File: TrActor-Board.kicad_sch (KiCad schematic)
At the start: 24 parts, among them J3 GCT4720, J4 Batt, J5 NTC, SW1 Power, SW2 Reset, U3 LSM6DSO32, U6 USBLC6-2P6

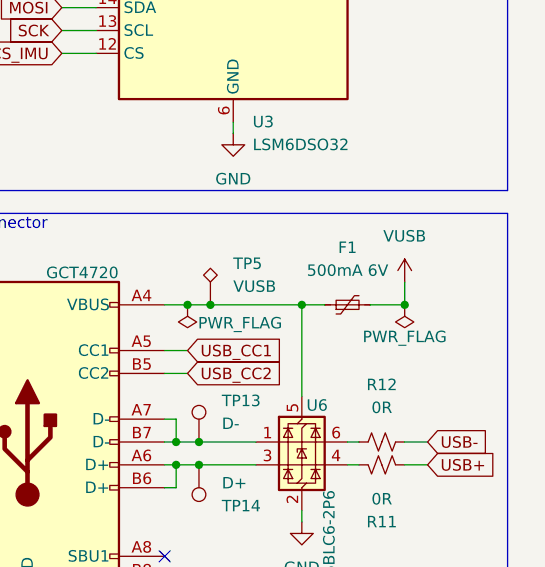
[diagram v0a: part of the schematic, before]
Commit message: routing started
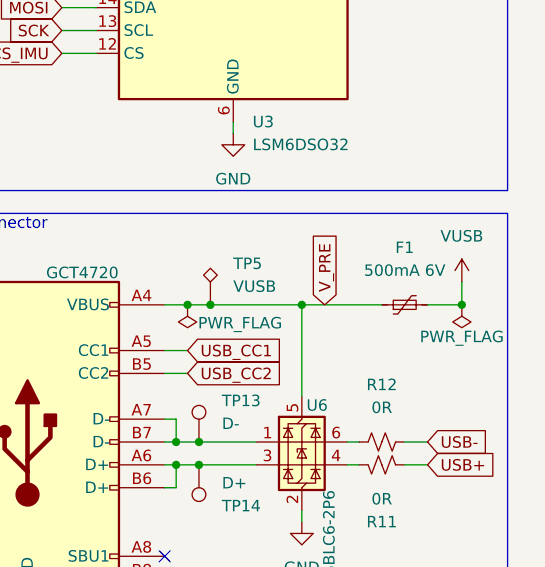
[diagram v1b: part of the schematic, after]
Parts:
- J5: footprint (none) -> Connector_JST:JST_SH_SM02B-SRSS-TB_1x02-1MP_P1.00mm_Horizontal
- JP1: footprint (none) -> Connector_PinHeader_2.54mm:PinHeader_1x02_P2.54mm_Vertical_SMD_Pin1Left
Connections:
- net V_PRE: now reaches F1.1, J3.A4 (VBUS), J3.A9 (VBUS), J3.B4 (VBUS), J3.B9 (VBUS), TP5.1, U6.5 (VBUS)
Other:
- moved on the sheet: F1
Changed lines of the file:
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@@
 	)
 	(junction
-		(at 252.73 82.55)
+		(at 259.08 82.55)
 		(diameter 0)
 		(color 0 0 0 0)
@@
 	)
 	(junction
+		(at 241.3 82.55)
+		(diameter 0)
+		(color 0 0 0 0)
+	)
+	(junction
 		(at 181.61 64.77)
 		(diameter 0)
@@
 	)
 	(junction
-		(at 241.3 82.55)
-		(diameter 0)
-		(color 0 0 0 0)
-	)
-	(junction
 		(at 191.77 64.77)
 		(diameter 0)
@@
 	(wire
 		(pts
-			(xy 252.73 82.55) (xy 248.92 82.55)
+			(xy 259.08 82.55) (xy 255.27 82.55)
 		)
 		(stroke
@@
 	(wire
 		(pts
-			(xy 243.84 82.55) (xy 241.3 82.55)
-		)
-		(stroke
-			(width 0)
-			(type default)
-		)
-	)
-	(wire
-		(pts
 			(xy 185.42 33.02) (xy 185.42 31.75)
 		)
@@
 	(wire
 		(pts
+			(xy 241.3 82.55) (xy 250.19 82.55)
+		)
+		(stroke
+			(width 0)
+			(type default)
+		)
+	)
+	(wire
+		(pts
 			(xy 172.72 78.74) (xy 176.53 78.74)
 		)
@@
 	(wire
 		(pts
-			(xy 252.73 80.01) (xy 252.73 82.55)
+			(xy 259.08 80.01) (xy 259.08 82.55)
 		)
 		(stroke
@@
 		)
 	)
+	(global_label "V_PRE"
+		(shape input)
+		(at 243.84 82.55 90)
+		(fields_autoplaced yes)
+		(effects
+			(font
+				(size 1.27 1.27)
+			)
+			(justify left)
+		)
+		(property "Intersheetrefs" "${INTERSHEET_REFS}"
+			(at 243.84 74.4738 90)
+			(hide yes)
+			(show_name no)
+			(do_not_autoplace no)
+			(effects
+				(font
+					(size 1.27 1.27)
+				)
+				(justify left)
+			)
+		)
+	)
 	(global_label "IMU_INT2"
 		(shape input)
@@
 	(symbol
 		(lib_id "power:VBUS")
-		(at 252.73 80.01 0)
+		(at 259.08 80.01 0)
 		(unit 1)
 		(body_style 1)
@@
 		(fields_autoplaced yes)
 		(property "Reference" "#PWR060"
-			(at 252.73 83.82 0)
+			(at 259.08 83.82 0)
 			(hide yes)
 			(show_name no)
@@
 		)
 		(property "Value" "VUSB"
-			(at 252.73 74.93 0)
+			(at 259.08 74.93 0)
 			(show_name no)
 			(do_not_autoplace no)
@@
 		)
 		(property "Footprint" ""
-			(at 252.73 80.01 0)
+			(at 259.08 80.01 0)
 			(hide yes)
 			(show_name no)
@@
 		)
 		(property "Datasheet" ""
-			(at 252.73 80.01 0)
+			(at 259.08 80.01 0)
 			(hide yes)
 			(show_name no)
@@
 		)
 		(property "Description" "Power symbol creates a global label with name \"VBUS\""
-			(at 252.73 80.01 0)
+			(at 259.08 80.01 0)
 			(hide yes)
 			(show_name no)
@@
 			)
 		)
-		(property "Footprint" ""
+		(property "Footprint" "Connector_JST:JST_SH_SM02B-SRSS-TB_1x02-1MP_P1.00mm_Horizontal"
 			(at 167.64 78.74 0)
 			(hide yes)
@@
 	(symbol
 		(lib_id "Device:Polyfuse_Small")
-		(at 246.38 82.55 90)
+		(at 252.73 82.55 90)
 		(unit 1)
 		(body_style 1)
@@
 		(fields_autoplaced yes)
 		(property "Reference" "F1"
-			(at 246.38 76.2 90)
+			(at 252.73 76.2 90)
 			(show_name no)
 			(do_not_autoplace no)
@@
 		)
 		(property "Value" "500mA 6V"
-			(at 246.38 78.74 90)
+			(at 252.73 78.74 90)
 			(show_name no)
 			(do_not_autoplace no)
@@
 		)
 		(property "Footprint" "Fuse:Fuse_0603_1608Metric"
-			(at 251.46 81.28 0)
+			(at 257.81 81.28 0)
 			(hide yes)
 			(show_name no)
@@
 		)
 		(property "Datasheet" ""
-			(at 246.38 82.55 0)
+			(at 252.73 82.55 0)
 			(hide yes)
 			(show_name no)
@@
 		)
 		(property "Description" "Resettable fuse, polymeric positive temperature coefficient, small symbol"
-			(at 246.38 82.55 0)
+			(at 252.73 82.55 0)
 			(hide yes)
 			(show_name no)
@@
 			)
 		)
-		(property "Footprint" ""
+		(property "Footprint" "Connector_PinHeader_2.54mm:PinHeader_1x02_P2.54mm_Vertical_SMD_Pin1Left"
 			(at 189.23 38.1 0)
 			(hide yes)
@@
 	(symbol
 		(lib_id "power:PWR_FLAG")
-		(at 252.73 82.55 0)
+		(at 259.08 82.55 0)
 		(mirror x)
 		(unit 1)
@@
 		(dnp no)
 		(property "Reference" "#FLG02"
-			(at 252.73 84.455 0)
+			(at 259.08 84.455 0)
 			(hide yes)
 			(show_name no)
@@
 		)
 		(property "Value" "PWR_FLAG"
-			(at 252.73 86.106 0)
+			(at 259.08 86.106 0)
 			(show_name no)
 			(do_not_autoplace no)
@@
 		)
 		(property "Footprint" ""
-			(at 252.73 82.55 0)
+			(at 259.08 82.55 0)
 			(hide yes)
 			(show_name no)
@@
 		)
 		(property "Datasheet" ""
-			(at 252.73 82.55 0)
+			(at 259.08 82.55 0)
 			(hide yes)
 			(show_name no)
@@
 		)
 		(property "Description" "Special symbol for telling ERC where power comes from"
-			(at 252.73 82.55 0)
+			(at 259.08 82.55 0)
 			(hide yes)
 			(show_name no)
